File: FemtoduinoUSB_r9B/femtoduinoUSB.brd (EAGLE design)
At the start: 20.7 x 15.2 mm, 29 parts, among them IC2 FT231XQ-R, U1 MIC5205

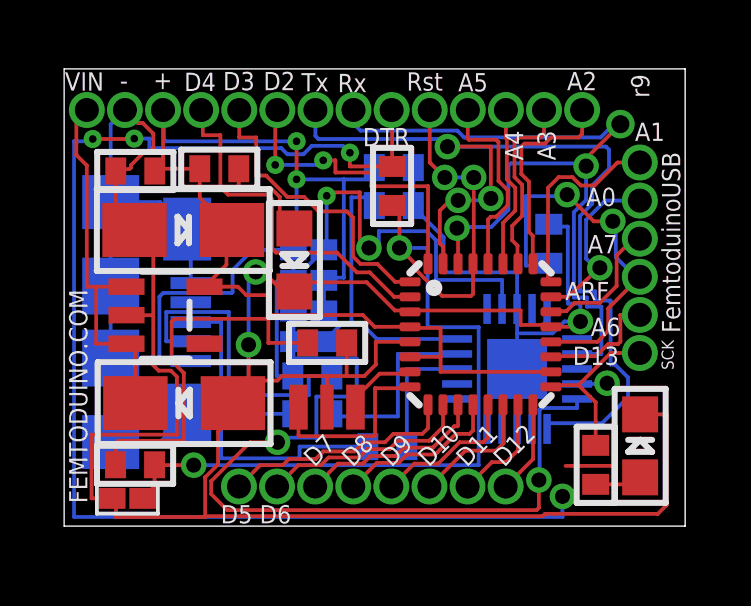
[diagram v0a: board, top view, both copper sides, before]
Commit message: Adding revision 9C
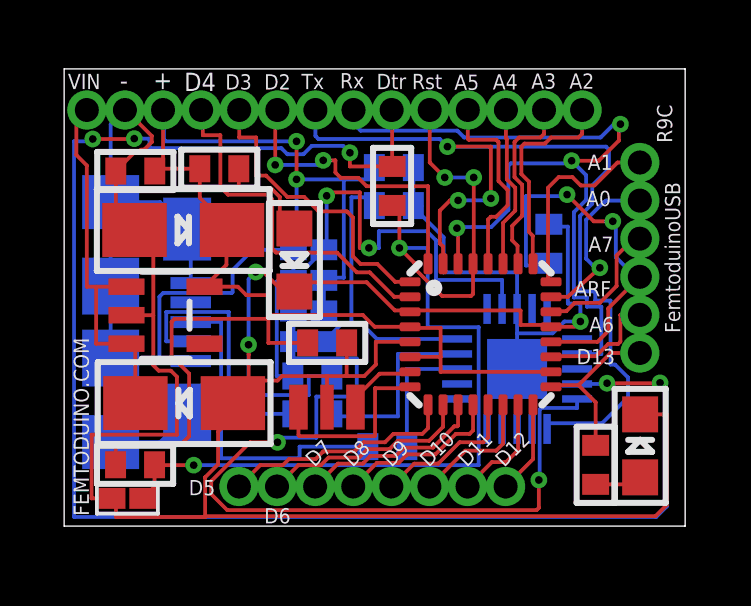
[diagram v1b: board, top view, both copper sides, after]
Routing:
- net DTR: track 48.6 -> 53.1 mm
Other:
- board text added: "Dtr"
- board text added: "R9C"
- board text removed: "DTR"
- board text removed: "SCK"
- board text removed: "r9"
